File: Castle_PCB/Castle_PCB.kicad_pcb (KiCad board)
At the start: 2 copper layers, 100 x 100 mm, 106 parts, among them J1 Conn_01x05_Pin, J2 Conn_01x02_Pin, Q1 NPN, U1 ESP32-DEVKITC, U2 74HC595, U3 74HC595, U6 LM35-LP

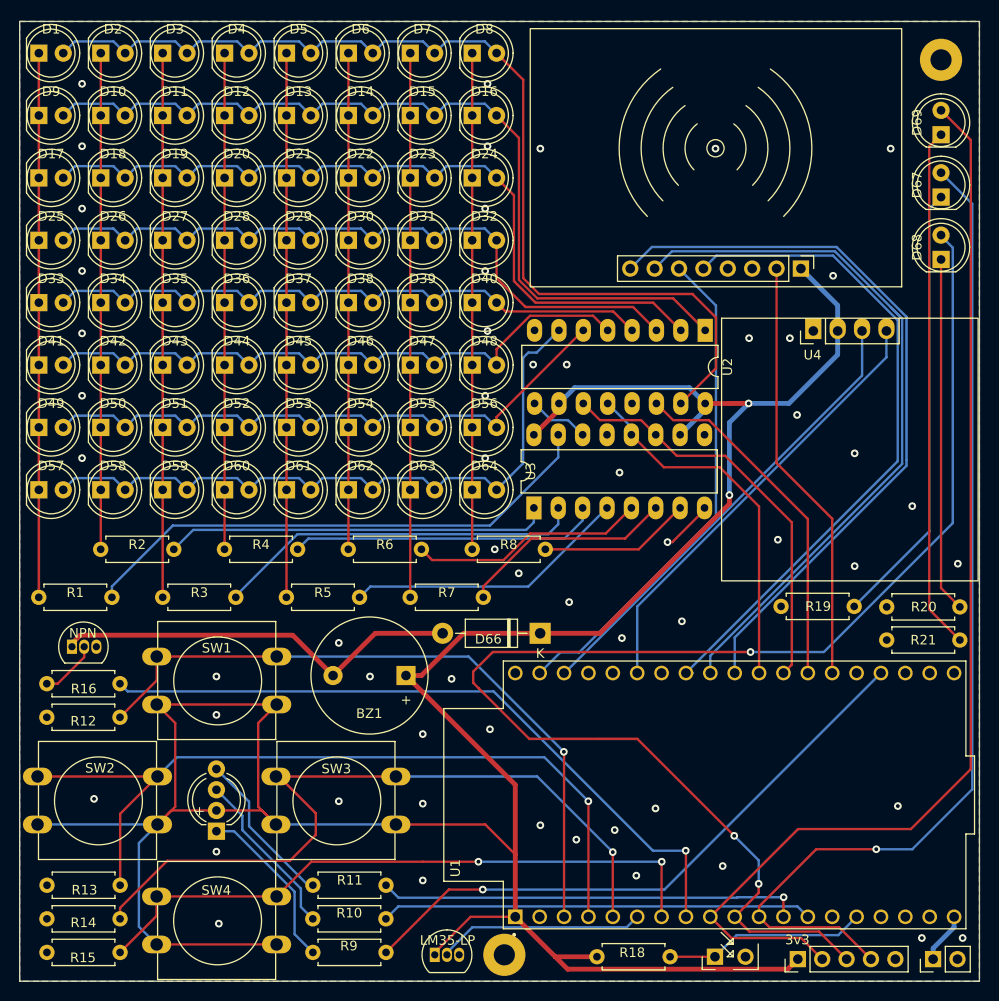
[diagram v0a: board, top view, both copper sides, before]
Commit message: pcb done!
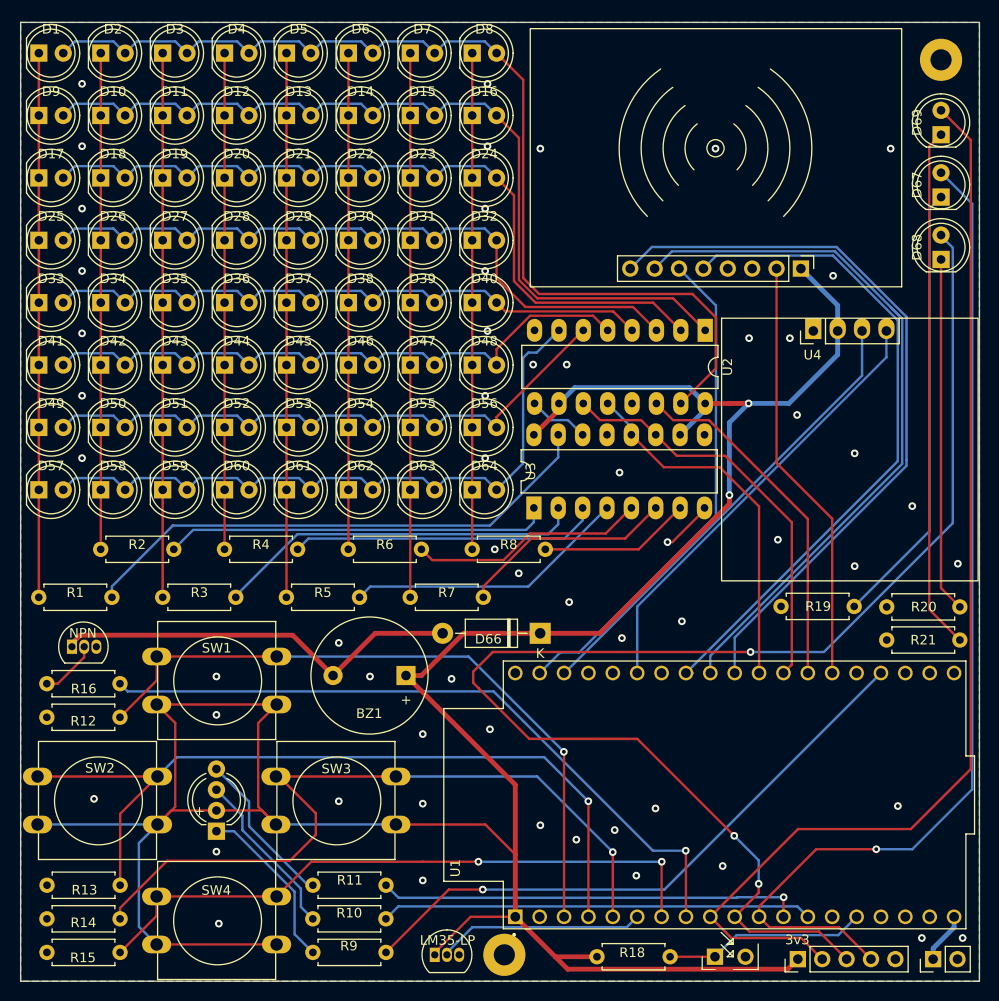
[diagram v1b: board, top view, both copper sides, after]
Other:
- board size 100 x 100 mm -> 99.9 x 99.9 mm
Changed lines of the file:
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@@
     (fp_arc (start 3.185339 20.793331) (mid -1.099323 13.44) (end 1.800824 5.438816)
       (stroke (width 0.1) (type default)) (layer "F.SilkS"))
-    (fp_arc (start 4.455339 18.88833) (mid 1.178719 13.214426) (end 3.41944 7.057432)
+    (fp_arc (start 4.455339 18.88833) (mid 1.178719 13.214427) (end 3.41944 7.057432)
       (stroke (width 0.1) (type default)) (layer "F.SilkS"))
     (fp_arc (start 5.725339 16.983331) (mid 3.456475 12.988879) (end 5.037785 8.675777)
@@
     )
   )
-  (gr_rect locked (start 100 50) (end 200 150)
+  (gr_rect (start 100.1 50.1) (end 200 150)
     (stroke (width 0.1) (type default)) (fill none) (layer "Edge.Cuts"))
   (gr_text "3v3" (at 179.75 146.27) (layer "F.SilkS")
@@
     (polygon
       (pts
-        (xy 100 50)
-        (xy 200 50)
+        (xy 100.1 50.1)
+        (xy 200 50.1)
         (xy 200 150)
-        (xy 100 150)
+        (xy 100.1 150)
       )
     )
